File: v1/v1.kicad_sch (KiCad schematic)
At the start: 7 parts, among them J1 Conn_02x22_Top_Bottom, U1 ESP32-S3-DevKitC, U2 DM-OLED096-636

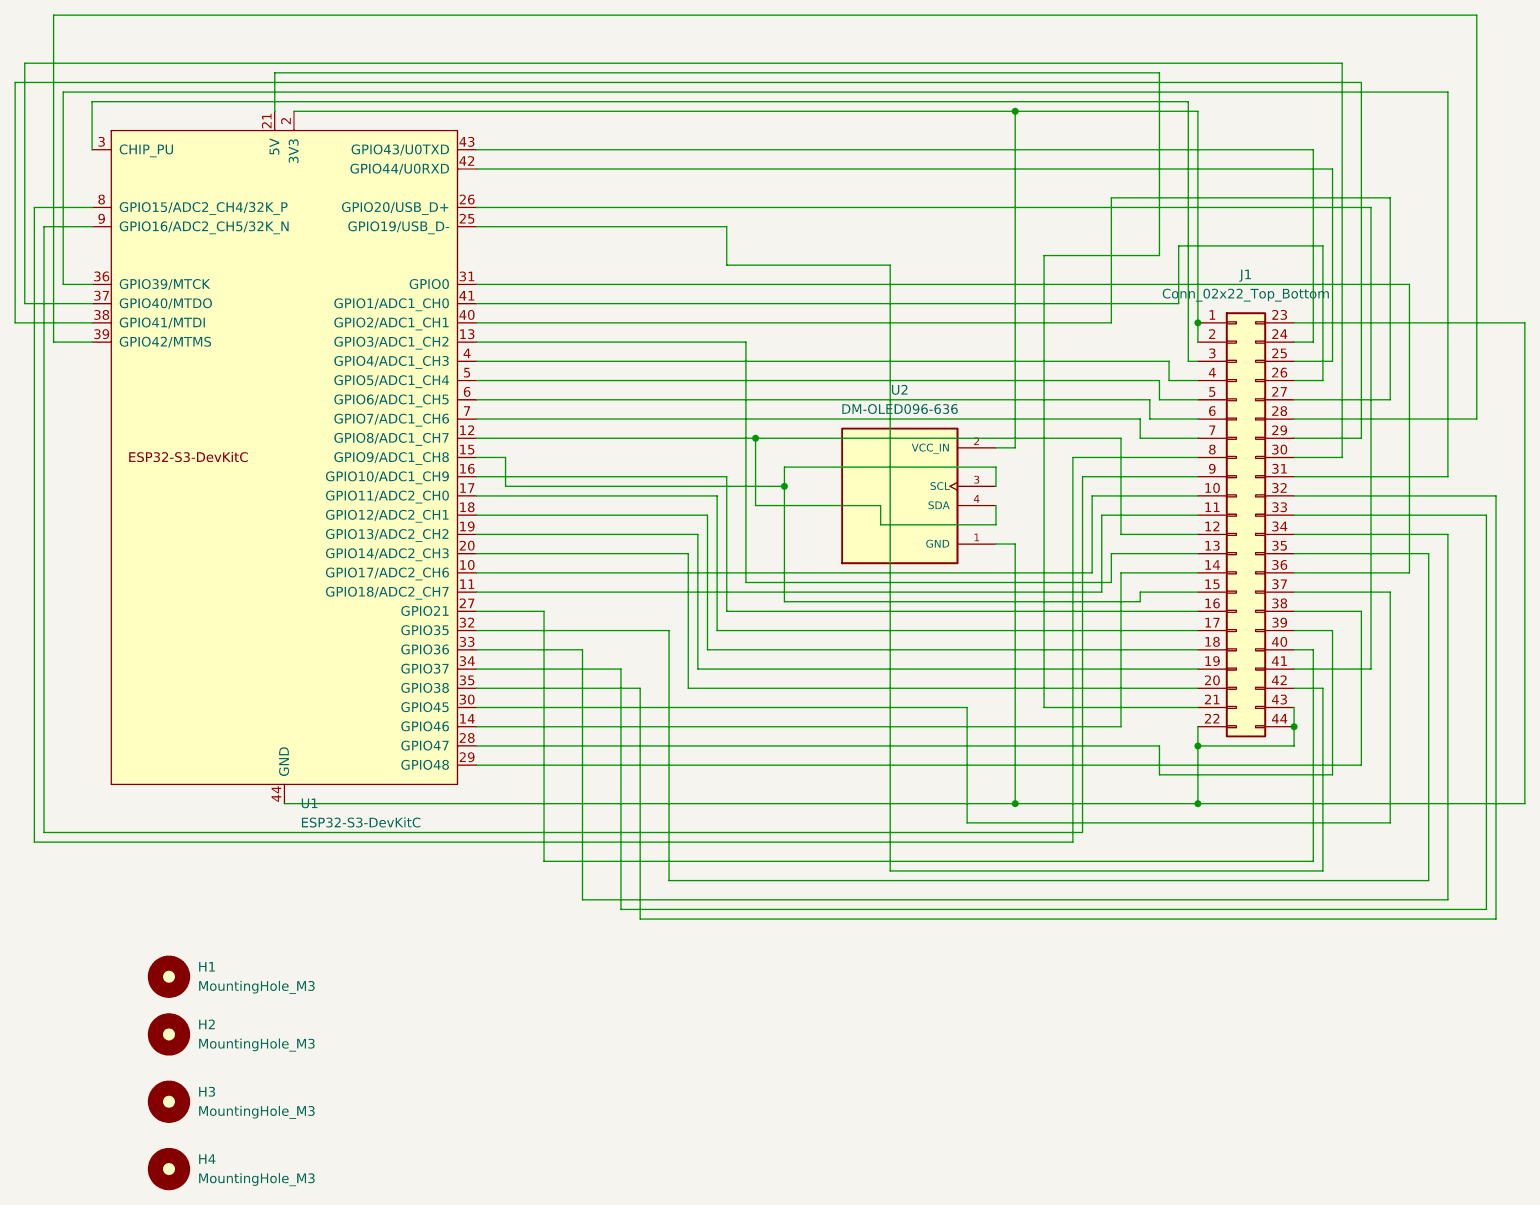
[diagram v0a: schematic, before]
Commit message: code, new pcb and bom
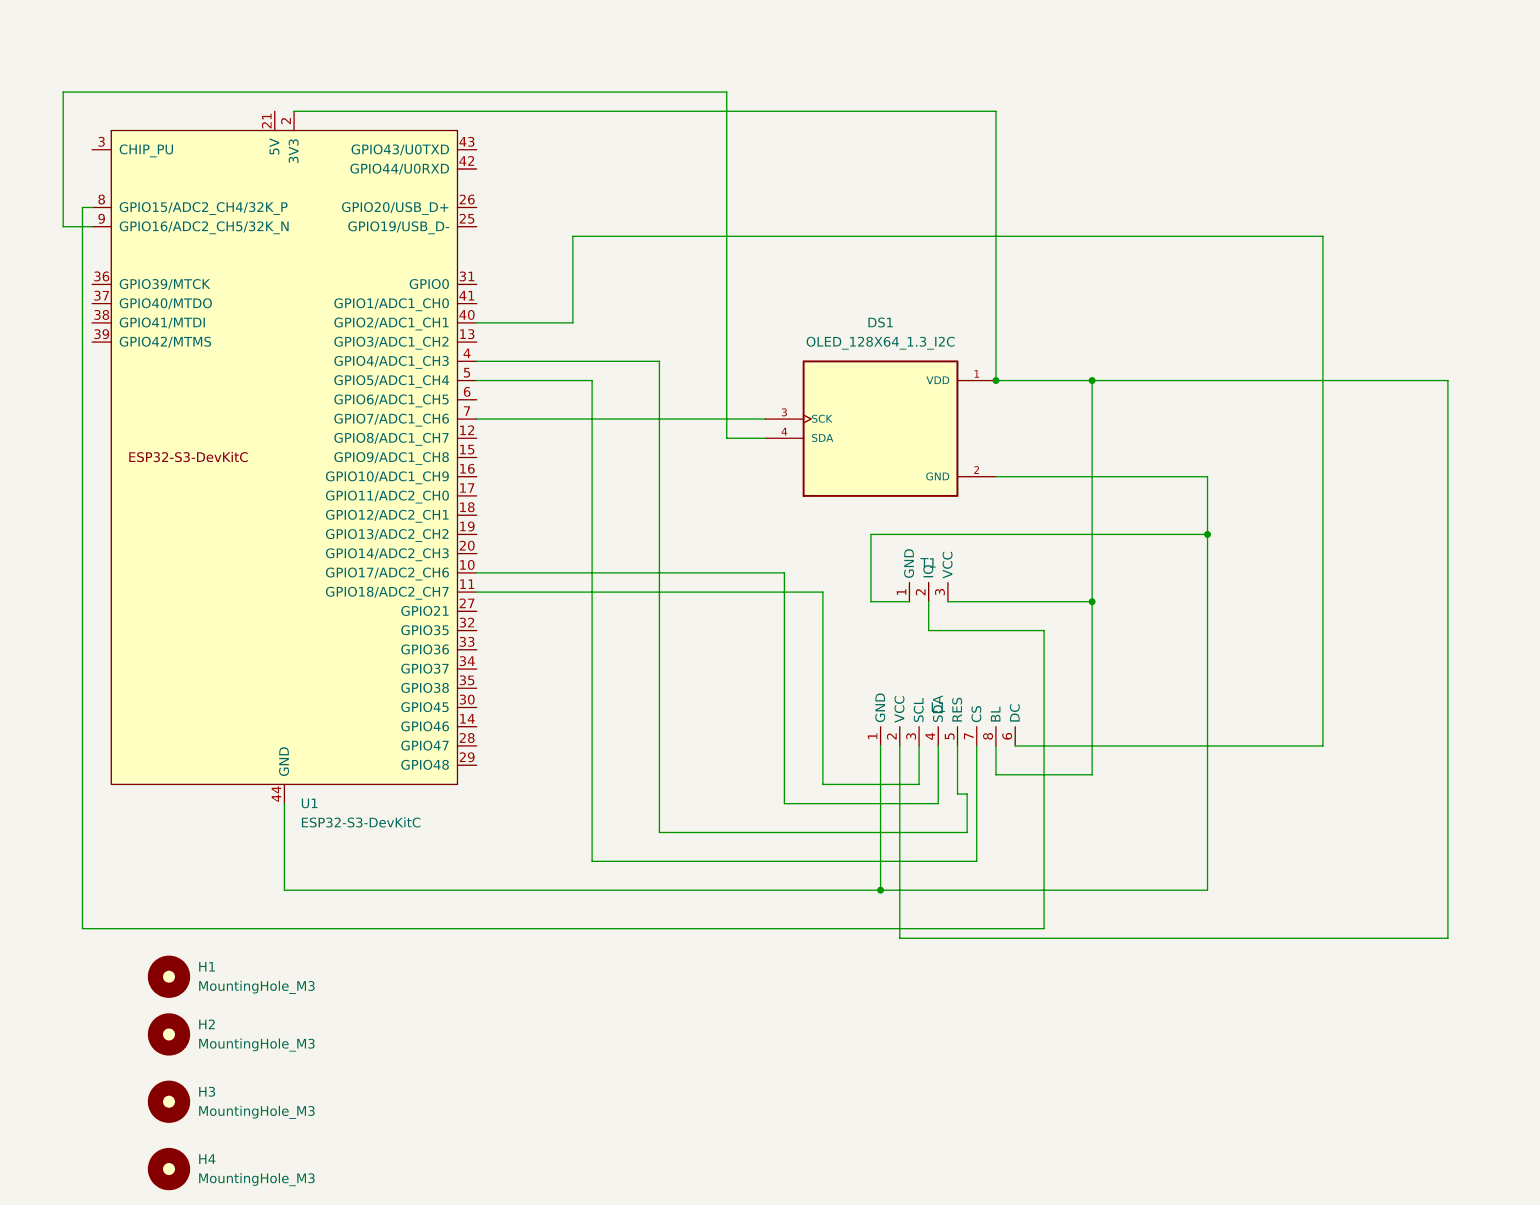
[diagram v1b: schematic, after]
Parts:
- removed J1: Conn_02x22_Top_Bottom, Connector_PinHeader_2.54mm:PinHeader_2x22_P2.54mm_Vertical, symbol Connector_Generic:Conn_02x22_Top_Bottom
- removed U2: DM-OLED096-636, Library:MODULE_DM-OLED096-636, symbol DM-OLED096-636:DM-OLED096-636
- added DS1: OLED_128X64_1.3_I2C, LCD_OLED_128X64_1.3_I2C:LCD_OLED_128X64_1.3_I2C, symbol OLED_128X64_1.3_I2C:OLED_128X64_1.3_I2C
- added L1: (no value), Connector_PinHeader_2.54mm:PinHeader_1x08_P2.54mm_Vertical, symbol New_Library:LCD_1
- added T1: (no value), Connector_PinHeader_2.54mm:PinHeader_1x03_P2.54mm_Vertical, symbol New_Library:_TTP223
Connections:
- net at U1.1 (3V3), U1.2 (3V3): now also DS1.1 (VDD), L1.2 (VCC), L1.8 (BL), T1.3 (VCC)
- net at U1.10 (GPIO17/ADC2_CH6): now also L1.4 (SDA)
- net at U1.11 (GPIO18/ADC2_CH7): now also L1.3 (SCL)
- net at U1.22 (GND), U1.23 (GND), U1.24 (GND)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: now also DS1.2 (GND), L1.1 (GND), T1.1 (GND)
- net at U1.40 (GPIO2/ADC1_CH1): now also L1.6 (DC)
- net at U1.4 (GPIO4/ADC1_CH3): now also L1.5 (RES)
- net at U1.5 (GPIO5/ADC1_CH4): now also L1.7 (CS)
- net at U1.7 (GPIO7/ADC1_CH6): now also DS1.3 (SCK)
- net at U1.8 (GPIO15/ADC2_CH4/32K_P): now also T1.2 (IO)
- net at U1.9 (GPIO16/ADC2_CH5/32K_N): now also DS1.4 (SDA)
